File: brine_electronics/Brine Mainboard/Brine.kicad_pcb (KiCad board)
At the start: 2 copper layers, 30.4 x 42.6 mm, 29 parts, among them J1 BATT, J2 BATT_CRG_GND, J3 BATT_CRG_BATT, J4 BATT_CRG_BATT, J5 BATT_CRG_GND, Q1 AO3407A, U1 XIAO-ESP32-S3-SMD, U2 VL53L1CXV0FY1, U3 LTC2954, U4 74AHCT1G125

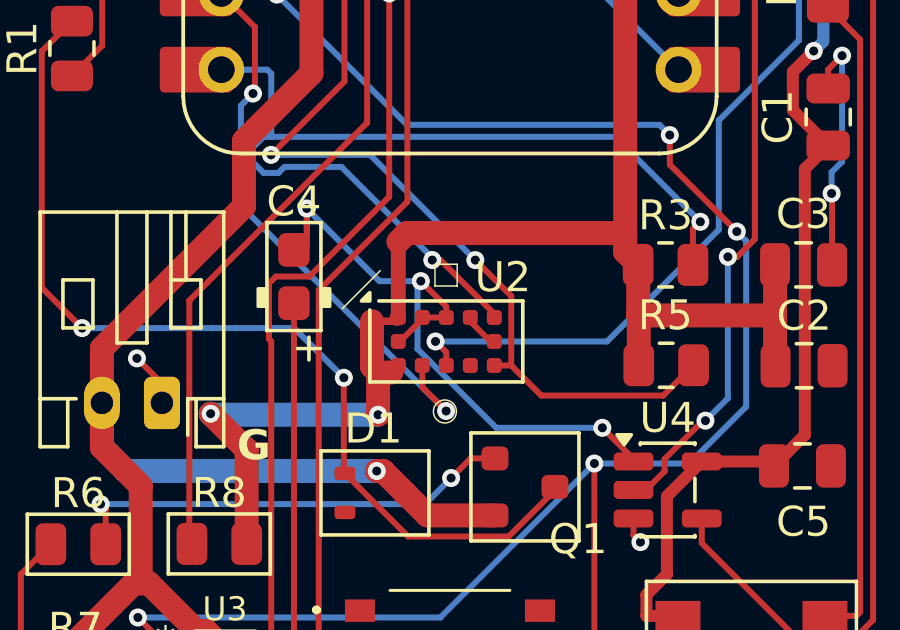
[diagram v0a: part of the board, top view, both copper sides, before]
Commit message: Updated distance sensor routing 📏
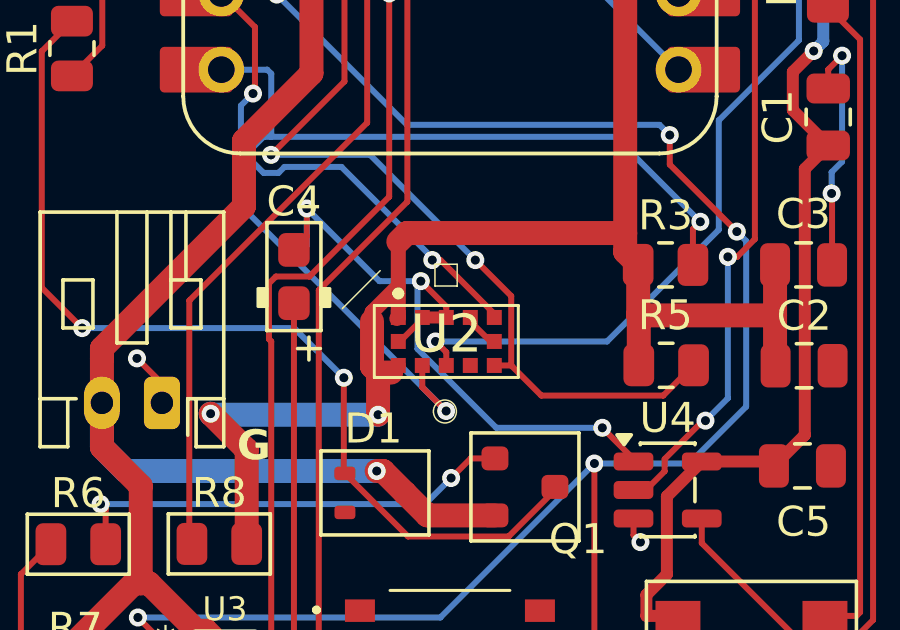
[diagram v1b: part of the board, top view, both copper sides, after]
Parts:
- U2: footprint Sensor_Distance:ST_VL53L1x -> VL53L1CXV0FY_1:VL53L1CXV0FY1
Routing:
- net +3.3V: track 66.1 -> 67.8 mm
